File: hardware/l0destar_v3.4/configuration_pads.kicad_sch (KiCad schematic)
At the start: 5 parts

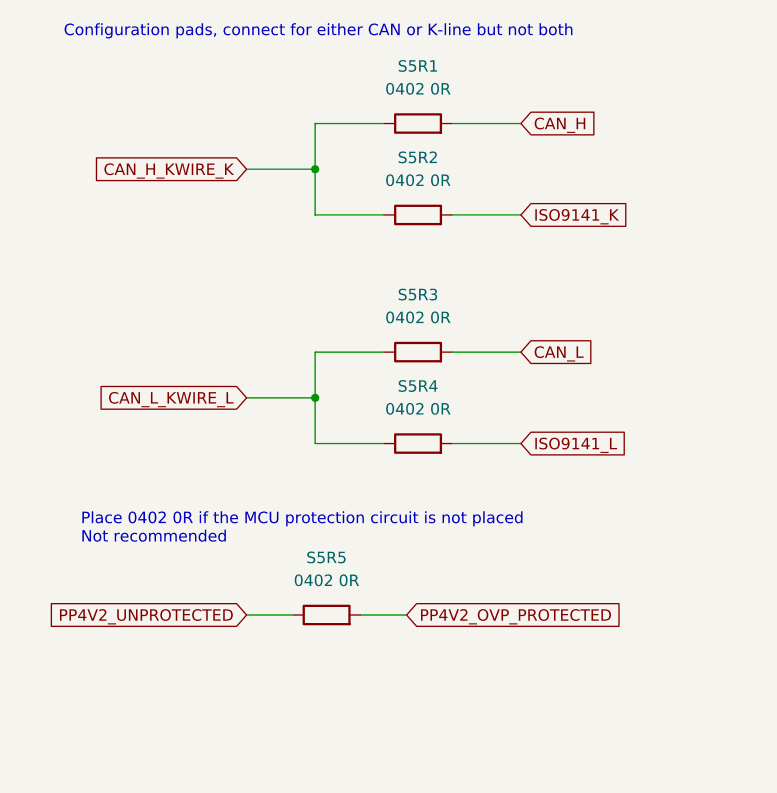
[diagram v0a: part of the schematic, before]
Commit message: doc updates
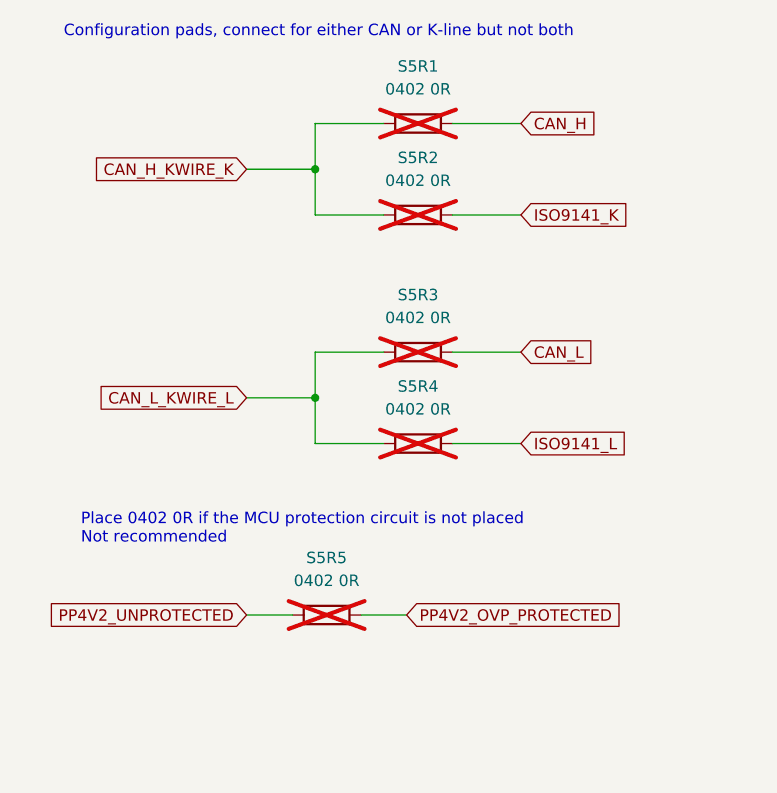
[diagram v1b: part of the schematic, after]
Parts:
- S5R1, S5R2, S5R3, S5R4, S5R5: now not fitted
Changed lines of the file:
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@@
 		(on_board yes)
 		(in_pos_files yes)
-		(dnp no)
+		(dnp yes)
 		(fields_autoplaced yes)
 		(property "Reference" "S5R3"
@@
 		(on_board yes)
 		(in_pos_files yes)
-		(dnp no)
+		(dnp yes)
 		(fields_autoplaced yes)
 		(property "Reference" "S5R1"
@@
 		(on_board yes)
 		(in_pos_files yes)
-		(dnp no)
+		(dnp yes)
 		(fields_autoplaced yes)
 		(property "Reference" "S5R4"
@@
 		(on_board yes)
 		(in_pos_files yes)
-		(dnp no)
+		(dnp yes)
 		(fields_autoplaced yes)
 		(property "Reference" "S5R5"
@@
 		(on_board yes)
 		(in_pos_files yes)
-		(dnp no)
+		(dnp yes)
 		(fields_autoplaced yes)
 		(property "Reference" "S5R2"
